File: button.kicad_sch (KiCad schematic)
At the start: 4 parts, among them SW1 SW_Push

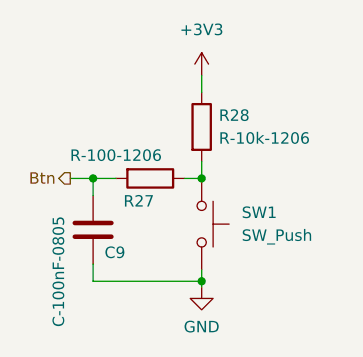
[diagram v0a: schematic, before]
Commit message: working on powers
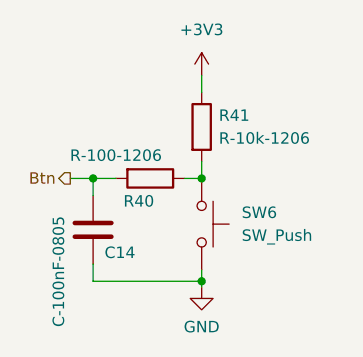
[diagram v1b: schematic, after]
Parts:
- renumbered C9 to C14, R27 to R40, R28 to R41, SW1 to SW6
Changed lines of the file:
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@@
     (effects (font (size 1.27 1.27)) (justify right))
   )
-  (symbol (lib_id "power:GND") (at 108.585 89.535 0) (unit 1)
+  (symbol (lib_id "power:GND") (at 108.585 89.535 0)
     (in_bom yes) (on_board yes) (fields_autoplaced)
-    (property "Reference" "#PWR030" (id 0) (at 108.585 95.885 0)
+    (property "Reference" "#PWR060" (id 0) (at 108.585 95.885 0)
       (effects (font (size 1.27 1.27)) hide)
     )
@@
     (pin "1")
   )
-  (symbol (lib_id "Switch:SW_Push") (at 108.585 82.55 270) (unit 1)
+  (symbol (lib_id "Switch:SW_Push") (at 108.585 82.55 270)
     (in_bom yes) (on_board yes) (fields_autoplaced)
-    (property "Reference" "SW1" (id 0) (at 113.03 81.2799 90)
+    (property "Reference" "SW6" (id 0) (at 113.03 81.2799 90)
       (effects (font (size 1.27 1.27)) (justify left))
     )
@@
     (pin "2")
   )
-  (symbol (lib_id "eurorack:R-10k-1206") (at 108.585 71.755 0) (unit 1)
+  (symbol (lib_id "eurorack:R-10k-1206") (at 108.585 71.755 0)
     (in_bom yes) (on_board yes) (fields_autoplaced)
-    (property "Reference" "R28" (id 0) (at 110.49 70.4849 0)
+    (property "Reference" "R41" (id 0) (at 110.49 70.4849 0)
       (effects (font (size 1.27 1.27)) (justify left))
     )
@@
     (pin "2")
   )
-  (symbol (lib_id "eurorack:C-100nF-0805") (at 96.52 83.185 0) (unit 1)
+  (symbol (lib_id "eurorack:C-100nF-0805") (at 96.52 83.185 0)
     (in_bom yes) (on_board yes)
-    (property "Reference" "C9" (id 0) (at 97.79 85.725 0)
+    (property "Reference" "C14" (id 0) (at 97.79 85.725 0)
       (effects (font (size 1.27 1.27)) (justify left))
     )
@@
     (pin "2")
   )
-  (symbol (lib_id "power:+3V3") (at 108.585 66.04 0) (unit 1)
+  (symbol (lib_id "power:+3V3") (at 108.585 66.04 0)
     (in_bom yes) (on_board yes) (fields_autoplaced)
-    (property "Reference" "#PWR029" (id 0) (at 108.585 69.85 0)
+    (property "Reference" "#PWR059" (id 0) (at 108.585 69.85 0)
       (effects (font (size 1.27 1.27)) hide)
     )
@@
     (pin "1")
   )
-  (symbol (lib_id "eurorack:R-100-1206") (at 102.87 77.47 270) (unit 1)
+  (symbol (lib_id "eurorack:R-100-1206") (at 102.87 77.47 270)
     (in_bom yes) (on_board yes)
-    (property "Reference" "R27" (id 0) (at 101.6 80.01 90))
+    (property "Reference" "R40" (id 0) (at 101.6 80.01 90))
     (property "Value" "R-100-1206" (id 1) (at 99.06 74.93 90))
     (property "Footprint" "Resistor_SMD:R_1206_3216Metric_Pad1.30x1.75mm_HandSolder" (id 2) (at 102.87 75.692 90)

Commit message: WIP
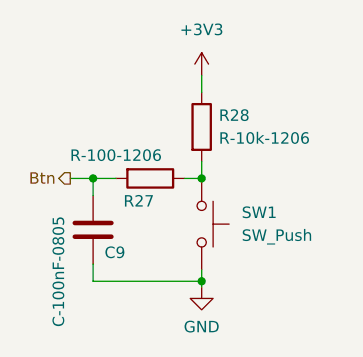
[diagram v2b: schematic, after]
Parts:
- renumbered C14 to C9, R40 to R27, R41 to R28, SW6 to SW1
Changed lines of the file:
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@@
     (effects (font (size 1.27 1.27)) (justify right))
   )
-  (symbol (lib_id "power:GND") (at 108.585 89.535 0)
+  (symbol (lib_id "power:GND") (at 108.585 89.535 0) (unit 1)
     (in_bom yes) (on_board yes) (fields_autoplaced)
-    (property "Reference" "#PWR060" (id 0) (at 108.585 95.885 0)
+    (property "Reference" "#PWR030" (id 0) (at 108.585 95.885 0)
       (effects (font (size 1.27 1.27)) hide)
     )
@@
     (pin "1")
   )
-  (symbol (lib_id "Switch:SW_Push") (at 108.585 82.55 270)
+  (symbol (lib_id "Switch:SW_Push") (at 108.585 82.55 270) (unit 1)
     (in_bom yes) (on_board yes) (fields_autoplaced)
-    (property "Reference" "SW6" (id 0) (at 113.03 81.2799 90)
+    (property "Reference" "SW1" (id 0) (at 113.03 81.2799 90)
       (effects (font (size 1.27 1.27)) (justify left))
     )
@@
     (pin "2")
   )
-  (symbol (lib_id "eurorack:R-10k-1206") (at 108.585 71.755 0)
+  (symbol (lib_id "eurorack:R-10k-1206") (at 108.585 71.755 0) (unit 1)
     (in_bom yes) (on_board yes) (fields_autoplaced)
-    (property "Reference" "R41" (id 0) (at 110.49 70.4849 0)
+    (property "Reference" "R28" (id 0) (at 110.49 70.4849 0)
       (effects (font (size 1.27 1.27)) (justify left))
     )
@@
     (pin "2")
   )
-  (symbol (lib_id "eurorack:C-100nF-0805") (at 96.52 83.185 0)
+  (symbol (lib_id "eurorack:C-100nF-0805") (at 96.52 83.185 0) (unit 1)
     (in_bom yes) (on_board yes)
-    (property "Reference" "C14" (id 0) (at 97.79 85.725 0)
+    (property "Reference" "C9" (id 0) (at 97.79 85.725 0)
       (effects (font (size 1.27 1.27)) (justify left))
     )
@@
     (pin "2")
   )
-  (symbol (lib_id "power:+3V3") (at 108.585 66.04 0)
+  (symbol (lib_id "power:+3V3") (at 108.585 66.04 0) (unit 1)
     (in_bom yes) (on_board yes) (fields_autoplaced)
-    (property "Reference" "#PWR059" (id 0) (at 108.585 69.85 0)
+    (property "Reference" "#PWR029" (id 0) (at 108.585 69.85 0)
       (effects (font (size 1.27 1.27)) hide)
     )
@@
     (pin "1")
   )
-  (symbol (lib_id "eurorack:R-100-1206") (at 102.87 77.47 270)
+  (symbol (lib_id "eurorack:R-100-1206") (at 102.87 77.47 270) (unit 1)
     (in_bom yes) (on_board yes)
-    (property "Reference" "R40" (id 0) (at 101.6 80.01 90))
+    (property "Reference" "R27" (id 0) (at 101.6 80.01 90))
     (property "Value" "R-100-1206" (id 1) (at 99.06 74.93 90))
     (property "Footprint" "Resistor_SMD:R_1206_3216Metric_Pad1.30x1.75mm_HandSolder" (id 2) (at 102.87 75.692 90)
